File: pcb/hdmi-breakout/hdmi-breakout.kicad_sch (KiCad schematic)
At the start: 5 parts, among them J1 Conn_01x09, J2 HDMI_A_1.4, J3 HDMI_A_1.4, J4 Conn_01x09

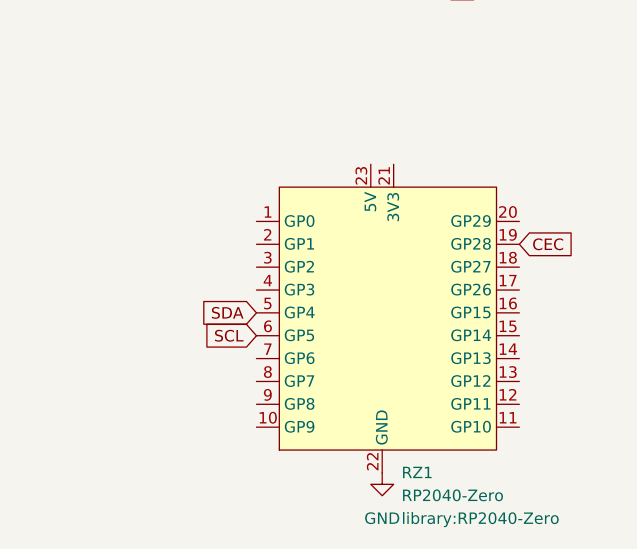
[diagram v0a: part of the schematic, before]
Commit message: update docs
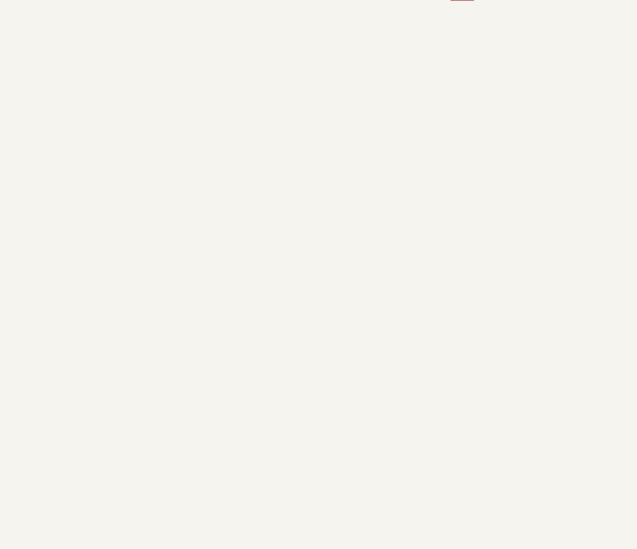
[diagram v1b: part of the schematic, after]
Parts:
- removed RZ1: RP2040-Zero, library:RP2040-Zero, symbol rp2040-zero:RP2040-Zero
